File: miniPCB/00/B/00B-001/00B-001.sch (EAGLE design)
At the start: 27 parts, among them U1 324

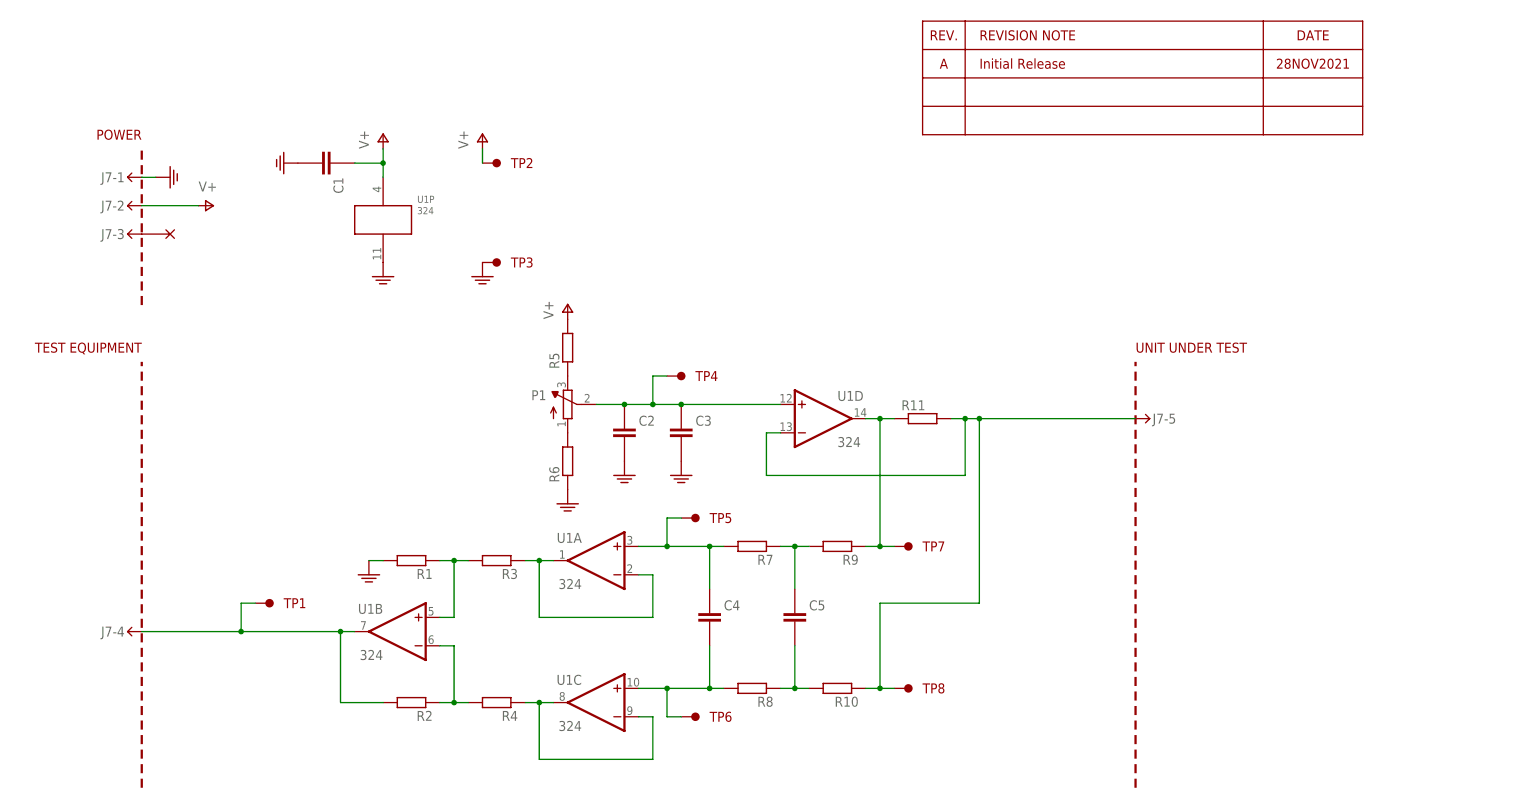
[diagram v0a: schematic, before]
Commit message: NM.23OCT2023
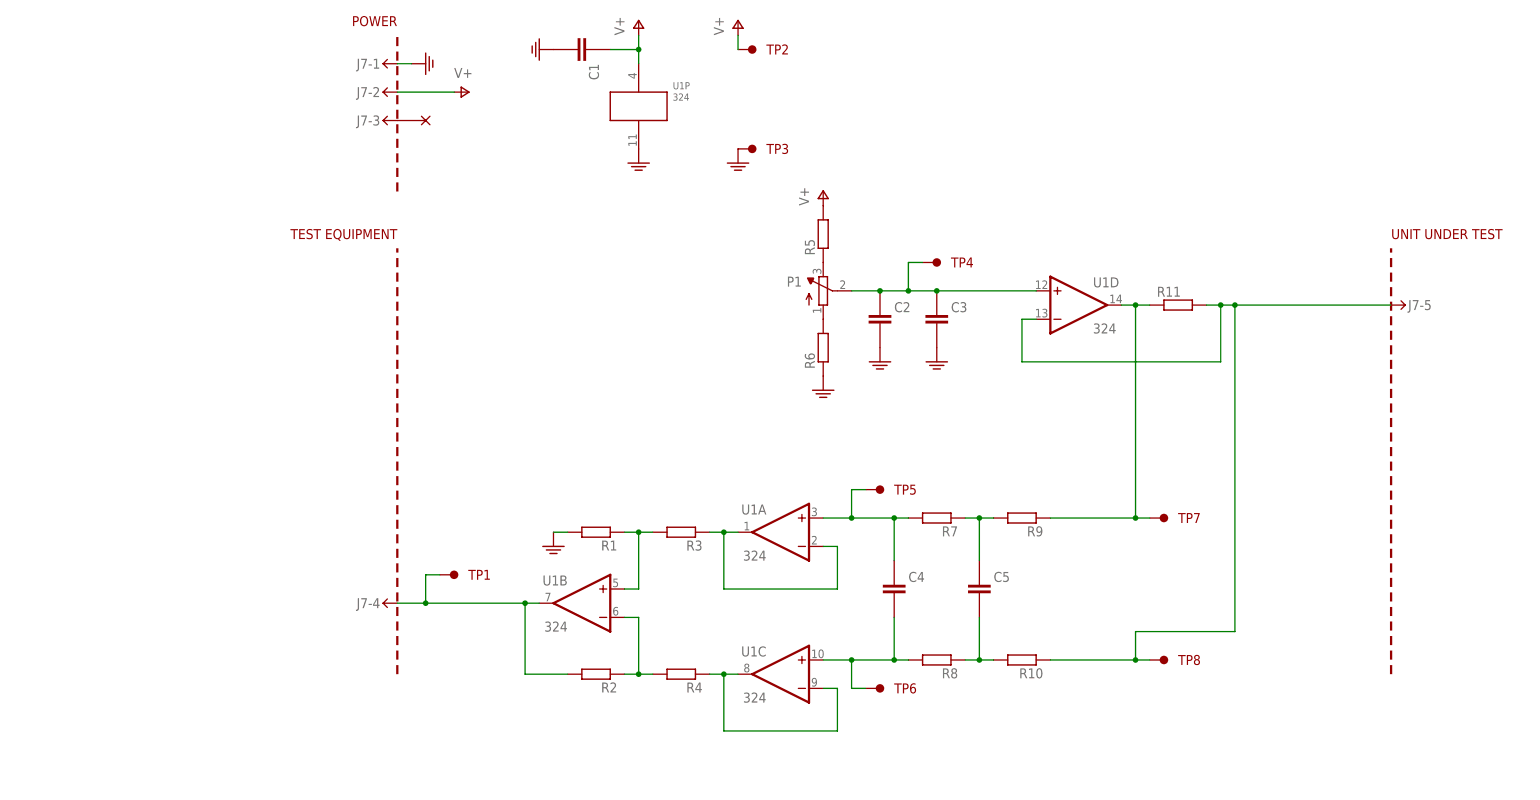
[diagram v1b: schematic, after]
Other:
- note removed: "28NOV2021"
- moved on the sheet: C1, C2, C3, C4, C5, J7-1, J7-2, J7-3, J7-4, J7-5, P1, R1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
